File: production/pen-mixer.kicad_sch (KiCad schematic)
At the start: 32 parts, among them J1 USB-C 16P, J2 BAT, J3 FSR, U1 ISP1807-LR, U2 LSM6DSV16X, U3 MCP73831T-2ACI/OT, U4 TPS7A0233DQN

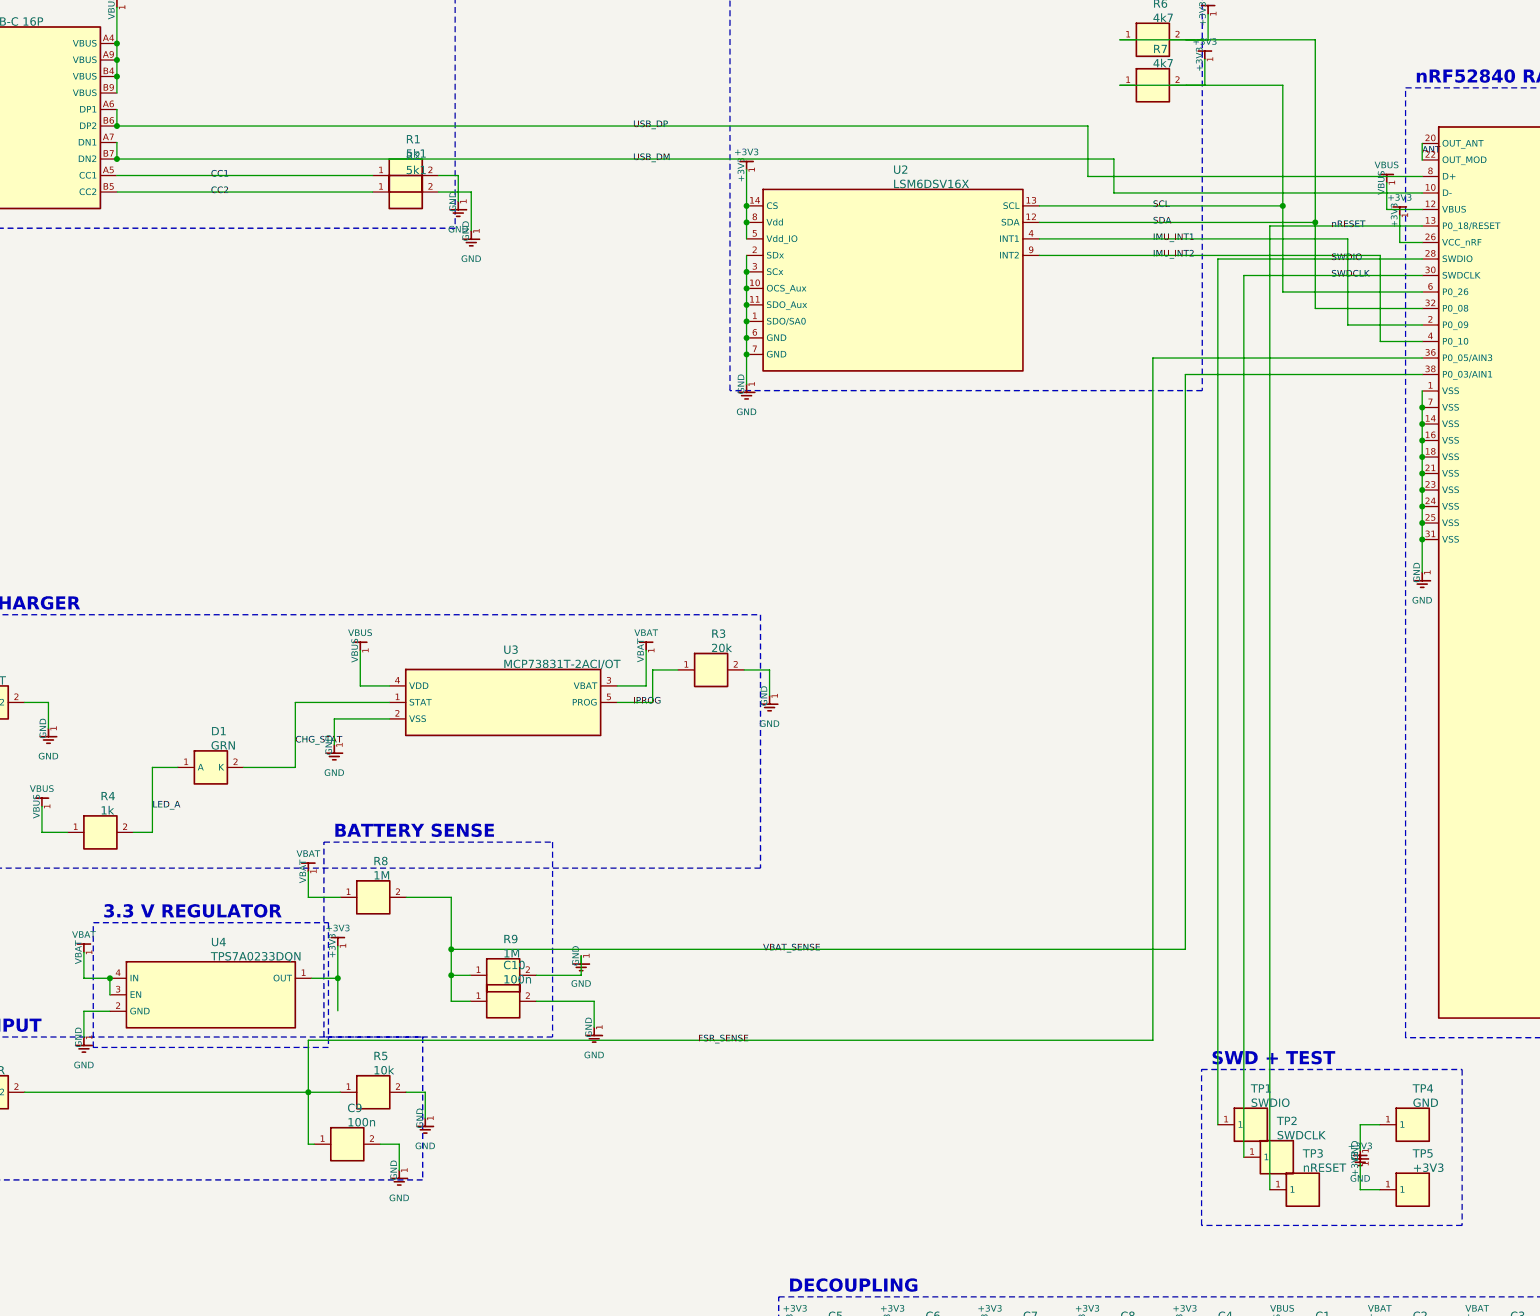
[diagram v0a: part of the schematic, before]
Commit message: wires in modules globals between
Claude-Session: https://claude.ai/code/session_01RCYT2QSY7BVZDeTyE9KrC4
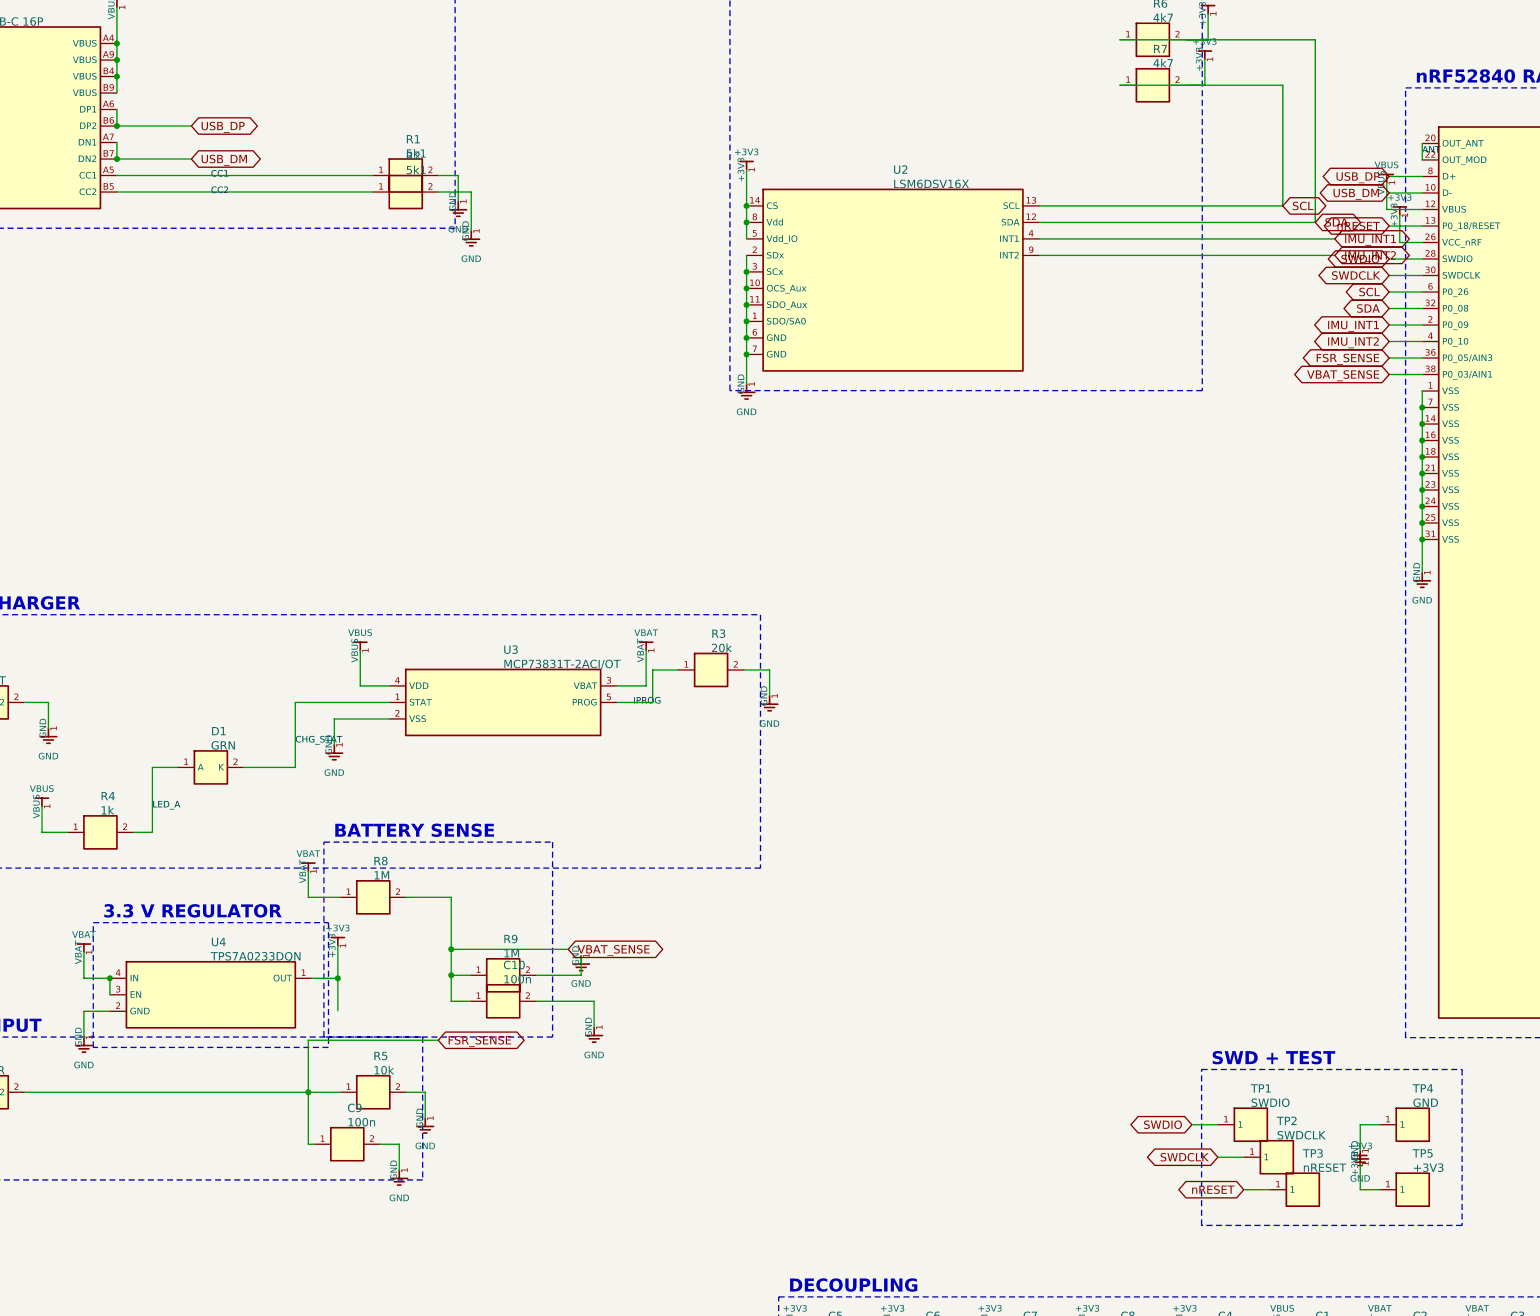
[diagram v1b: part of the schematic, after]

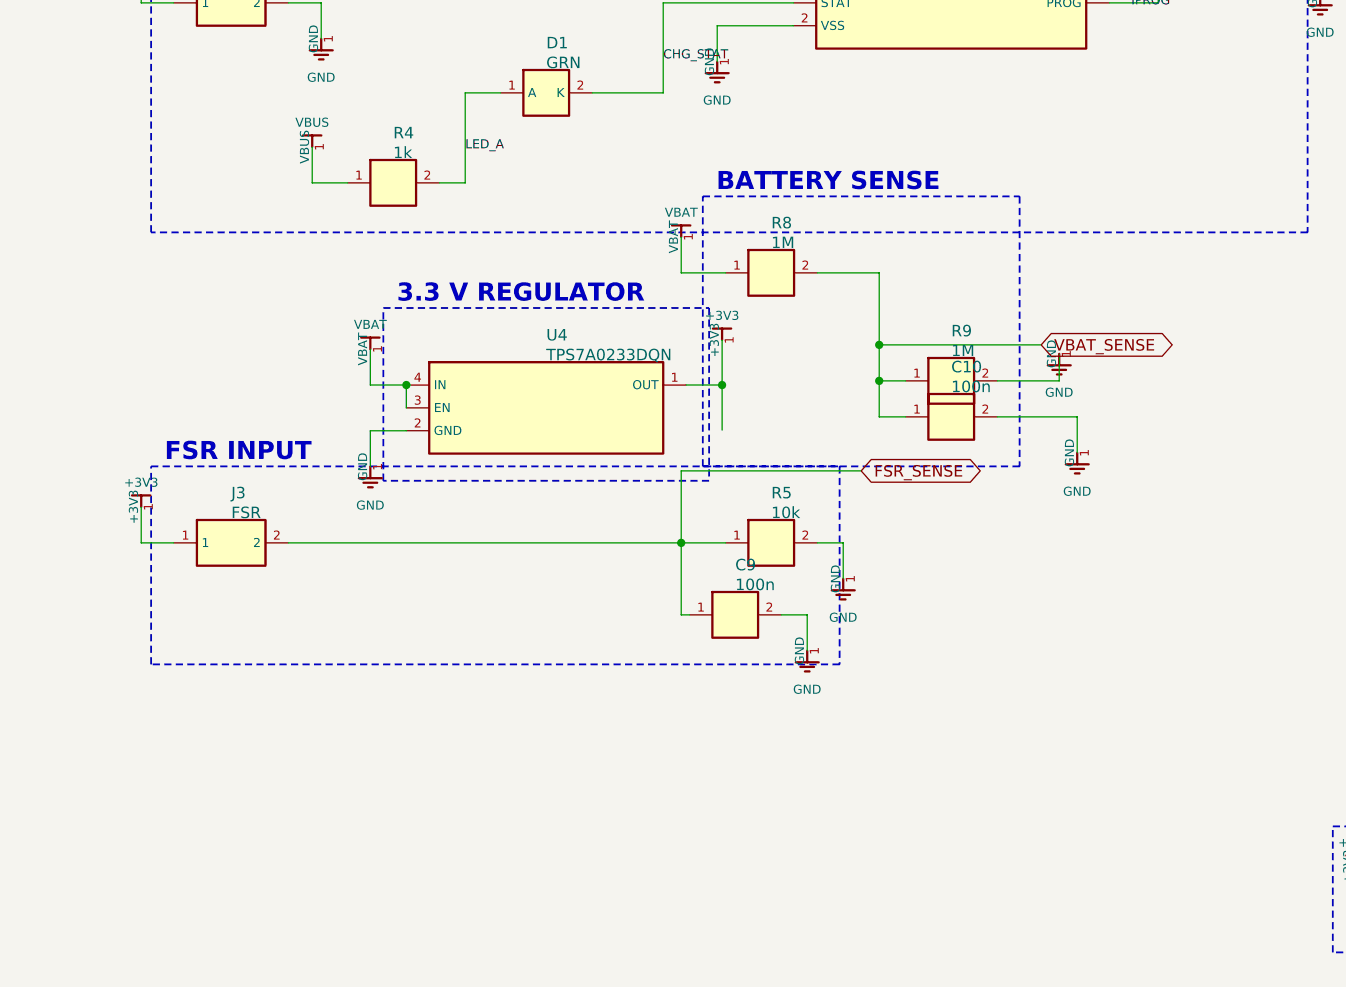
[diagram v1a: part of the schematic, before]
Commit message: arrange modules remove pours
Claude-Session: https://claude.ai/code/session_01RCYT2QSY7BVZDeTyE9KrC4
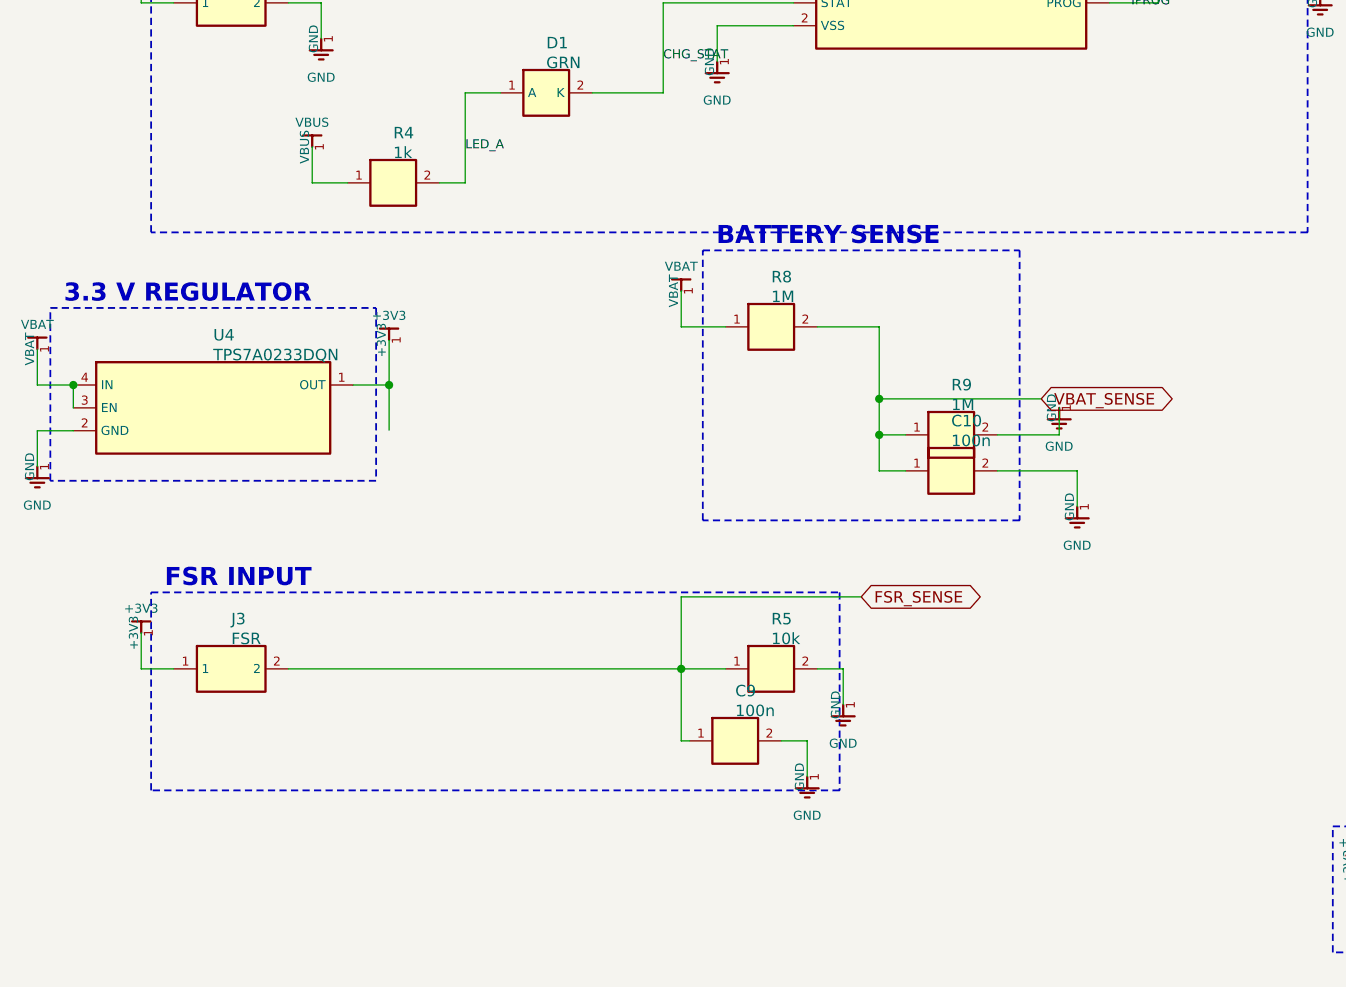
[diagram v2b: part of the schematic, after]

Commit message: stock symbols full route zero unrouted
Claude-Session: https://claude.ai/code/session_01RCYT2QSY7BVZDeTyE9KrC4
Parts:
- removed C1, C2: 4u7, Capacitor_SMD:C_0402_1005Metric, symbol pen-mixer:C
- removed C10, C5, C7, C8, C9: 100n, Capacitor_SMD:C_0402_1005Metric, symbol pen-mixer:C
- removed C3, C4: 1u, Capacitor_SMD:C_0402_1005Metric, symbol pen-mixer:C
- removed C6: 10u, Capacitor_SMD:C_0402_1005Metric, symbol pen-mixer:C
- removed D1: GRN, LED_SMD:LED_0402_1005Metric, symbol pen-mixer:LED
- removed J1: USB-C 16P, Connector_USB:USB_C_Receptacle_G-Switch_GT-USB-7010ASV, symbol pen-mixer:USB_C
- removed J2: BAT, pen-mixer:SolderPad_1.2x2.0mm, symbol pen-mixer:PAD2
- removed J3: FSR, pen-mixer:SolderPad_1.2x2.0mm, symbol pen-mixer:PAD2
- removed R1, R2: 5k1, Resistor_SMD:R_0402_1005Metric, symbol pen-mixer:R
- removed R3: 20k, Resistor_SMD:R_0402_1005Metric, symbol pen-mixer:R
- removed R4: 1k, Resistor_SMD:R_0402_1005Metric, symbol pen-mixer:R
- removed R5: 10k, Resistor_SMD:R_0402_1005Metric, symbol pen-mixer:R
- removed R6, R7: 4k7, Resistor_SMD:R_0402_1005Metric, symbol pen-mixer:R
- removed R8, R9: 1M, Resistor_SMD:R_0402_1005Metric, symbol pen-mixer:R
- removed TP1: SWDIO, pen-mixer:TestPad_1.0mm, symbol pen-mixer:TP
- removed TP2: SWDCLK, pen-mixer:TestPad_1.0mm, symbol pen-mixer:TP
- removed TP3: nRESET, pen-mixer:TestPad_1.0mm, symbol pen-mixer:TP
- removed TP4: GND, pen-mixer:TestPad_1.0mm, symbol pen-mixer:TP
- removed TP5: +3V3, pen-mixer:TestPad_1.0mm, symbol pen-mixer:TP
- removed U1: ISP1807-LR, pen-mixer:ISP1807_LGA78_8x8mm, symbol pen-mixer:ISP1807
- removed U2: LSM6DSV16X, Package_LGA:LGA-14_3x2.5mm_P0.5mm_LayoutBorder3x4y, symbol pen-mixer:LSM6DSV16X
- removed U3: MCP73831T-2ACI/OT, Package_TO_SOT_SMD:SOT-23-5, symbol pen-mixer:MCP73831
- removed U4: TPS7A0233DQN, Package_SON:Texas_X2SON-4_1x1mm_P0.65mm, symbol pen-mixer:TPS7A02
- added C1, C2: 4u7, Capacitor_SMD:C_0402_1005Metric, symbol Device:C
- added C10, C5, C7, C8, C9: 100n, Capacitor_SMD:C_0402_1005Metric, symbol Device:C
- added C3, C4: 1u, Capacitor_SMD:C_0402_1005Metric, symbol Device:C
- added C6: 10u, Capacitor_SMD:C_0402_1005Metric, symbol Device:C
- added D1: GRN, LED_SMD:LED_0402_1005Metric, symbol Device:LED
- added J1: USB-C 16P, Connector_USB:USB_C_Receptacle_G-Switch_GT-USB-7010ASV, symbol Connector:USB_C_Receptacle_USB2.0_16P
- added J2: BAT, pen-mixer:SolderPad_1.2x2.0mm, symbol Connector_Generic:Conn_01x02
- added J3: FSR, pen-mixer:SolderPad_1.2x2.0mm, symbol Connector_Generic:Conn_01x02
- added R1, R2: 5k1, Resistor_SMD:R_0402_1005Metric, symbol Device:R
- added R3: 20k, Resistor_SMD:R_0402_1005Metric, symbol Device:R
- added R4: 1k, Resistor_SMD:R_0402_1005Metric, symbol Device:R
- added R5: 10k, Resistor_SMD:R_0402_1005Metric, symbol Device:R
- added R6, R7: 4k7, Resistor_SMD:R_0402_1005Metric, symbol Device:R
- added R8, R9: 1M, Resistor_SMD:R_0402_1005Metric, symbol Device:R
- added TP1: SWDIO, pen-mixer:TestPad_1.0mm, symbol Connector:TestPoint
- added TP2: SWDCLK, pen-mixer:TestPad_1.0mm, symbol Connector:TestPoint
- added TP4: GND, pen-mixer:TestPad_1.0mm, symbol Connector:TestPoint
- added TP5: +3V3, pen-mixer:TestPad_1.0mm, symbol Connector:TestPoint
- added U1: ISP1807-LR, pen-mixer:ISP1807-LR, symbol ISP1807:ISP1807-LR
- added U2: LSM6DS3TR-C, Package_LGA:LGA-14_3x2.5mm_P0.5mm_LayoutBorder3x4y, symbol Sensor_Motion:LSM6DS3
- added U3: MCP73831T-2ACI/OT, Package_TO_SOT_SMD:SOT-23-5, symbol Battery_Management:MCP73831-2-OT
- added U4: TPS7A0533PDBV, Package_TO_SOT_SMD:SOT-23-5, symbol Regulator_Linear:TPS7A0533PDBV
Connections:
- net +3V3: now also C4.1, C5.1, C6.1, C7.1, C8.1, J3.1 (Pin_1), R6.2, R7.2, TP5.1, U1.26 (VCC_NRF), U2.12 (CS), U2.5 (VDDIO), U2.8 (VDD), U4.5 (OUT)
- net ANT: now also U1.20 (OUT_ANT), U1.22 (OUT_MOD)
- net CC1: now also J1.A5 (CC1), R1.1
- net CC2: now also J1.B5 (CC2), R2.1
- net CHG_STAT: now also D1.1 (K), U3.1 (STAT)
- net FSR_SENSE: now also C9.1, J3.2 (Pin_2), R5.1, U1.36 (P0.05/AIN3)
- net GND: now also C1.2, C10.2, C2.2, C3.2, C4.2, C5.2, C6.2, C7.2, C8.2, C9.2, J1.A1 (GND), J1.A12 (GND), J1.B1 (GND), J1.B12 (GND), J1.SH (SHIELD), J2.2 (Pin_2), R1.2, R2.2, R3.2, R5.2, R9.2, TP4.1, U1.1 (VSS@10), U1.14 (VSS@2), U1.16 (VSS@3), U1.18 (VSS@4), U1.21 (VSS@5), U1.23 (VSS@1), U1.24 (VSS@9), U1.25 (VSS@7), U1.31 (VSS@6), U1.7 (VSS@8), U2.1 (SDO/SA0), U2.2 (SDX), U2.3 (SCX), U2.6 (GND), U2.7 (GND), U3.2 (V_{SS}), U4.2 (GND)
- net IMU_INT1: now also U1.2 (P0.09/NFC1), U2.4 (INT1)
- net IMU_INT2: now also U1.4 (P0.10/NFC2), U2.9 (INT2)
- net IPROG: now also R3.1, U3.5 (PROG)
- net LED_A: now also D1.2 (A), R4.2
- net SWDCLK: now also TP2.1, U1.30 (SWDCLK)
- net SWDIO: now also TP1.1, U1.28 (SWDIO)
- net USB_DM: now also J1.A7 (D-), J1.B7 (D-), U1.10 (D-)
- net USB_DP: now also J1.A6 (D+), J1.B6 (D+), U1.8 (D+)
- net VBAT: now also C2.1, C3.1, J2.1 (Pin_1), R8.1, U3.3 (V_{BAT}), U4.1 (IN), U4.3 (EN)
- net VBAT_SENSE: now also C10.1, R8.2, R9.1, U1.38 (P0.03/AIN1)
- net VBUS: now also C1.1, J1.A4 (VBUS), J1.A9 (VBUS), J1.B4 (VBUS), J1.B9 (VBUS), R4.1, U1.12 (VBUS), U3.4 (V_{DD})
- new net SCL: R7.1, U1.6 (P0.26), U2.13 (SCL)
- new net SDA: R6.1, U1.32 (P0.08), U2.14 (SDA)
- no-connect marks 53 -> 59

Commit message: user layout radio module tidy
Claude-Session: https://claude.ai/code/session_01RCYT2QSY7BVZDeTyE9KrC4
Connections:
- net USB_DP is gone; now on net USB_DM: J1.A6 (D+), J1.B6 (D+), U1.8 (D+)
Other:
- moved on the sheet: C1, C10, C2, C3, C4, C5, C6, C7, C8, C9, D1, J1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
